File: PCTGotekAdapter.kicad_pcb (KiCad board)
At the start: 2 copper layers, 114.3 x 55.9 mm, 21 parts, among them J1 Conn_02x17_Odd_Even, J2 Conn_2Rows-19Pins, J3 Conn_2Rows-19Pins, J4 Conn_02x17_Odd_Even, J5 Conn_01x04_Pin, J6 Conn_01x04_Pin, U1 SN74LS138N, U2 SN7407N

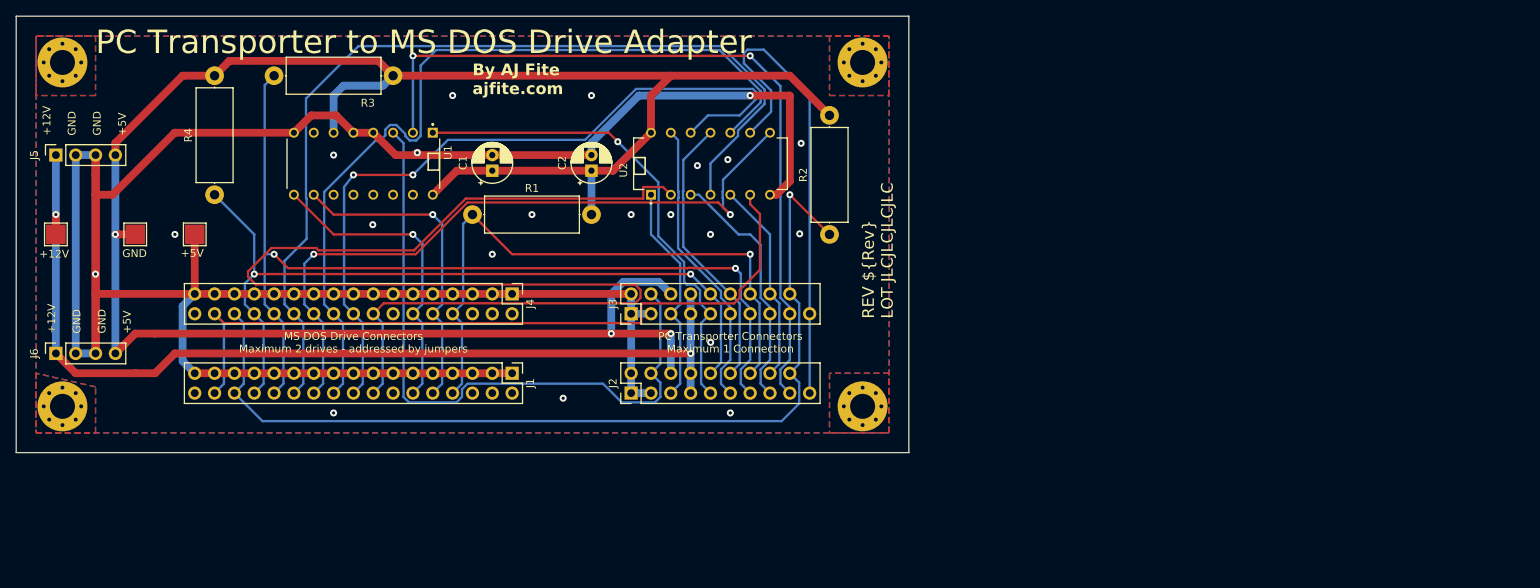
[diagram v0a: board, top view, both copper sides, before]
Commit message: First pass at REV B
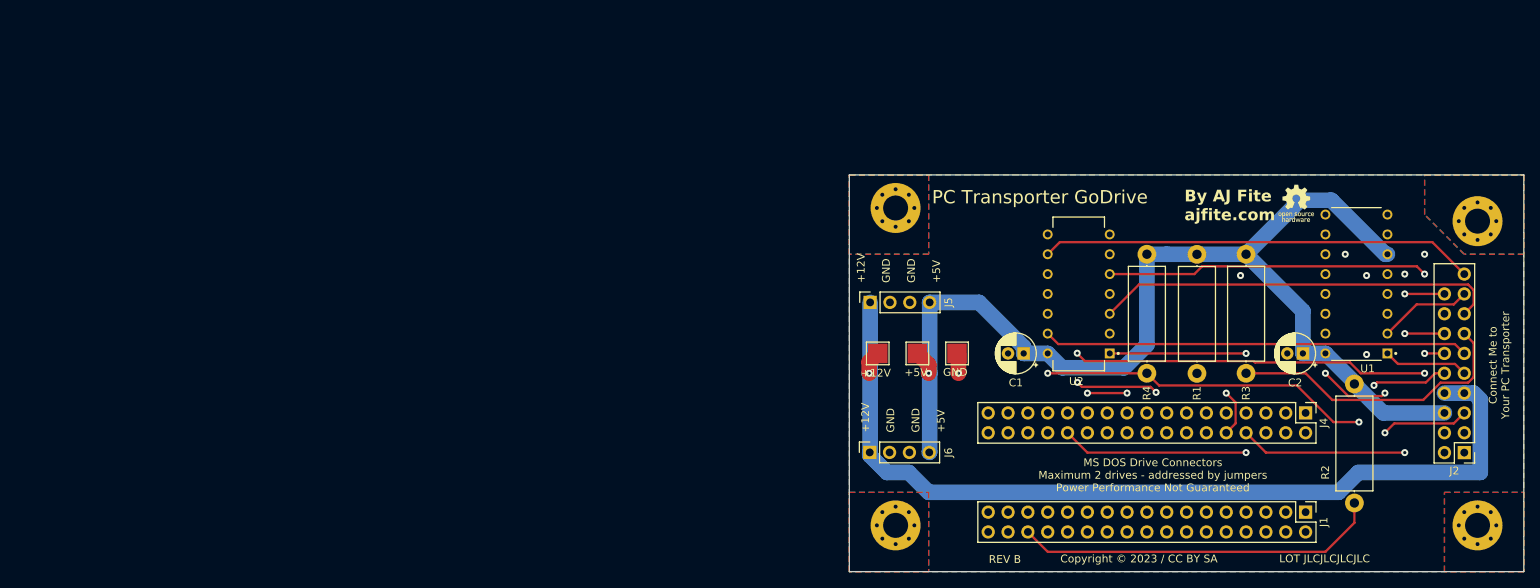
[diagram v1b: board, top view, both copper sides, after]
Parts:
- removed J3: Conn_2Rows-19Pins, Connector_PinHeader_2.54mm:PinHeader_2x10_P2.54mm_Vertical
- moved R3 130.2 mm to (175.3, 99.1), turned to 90 degrees
- moved U1 128.1 mm to (189.4, 87.6), turned to 180 degrees
- moved R4 121.5 mm to (162.6, 99.1)
- moved H1 108.3 mm to (130.4, 77.9)
- moved H2 107.8 mm to (130.4, 118.5)
- moved J2 107.0 mm to (203.2, 109.2), turned to 180 degrees
- moved TP1 106.3 mm to (128.1, 96.5)
- moved J5 106.0 mm to (127.1, 90.0)
- moved J6 105.0 mm to (127.1, 109.2)
- moved J1 103.1 mm to (182.9, 116.8)
- moved J4 102.7 mm to (182.9, 104.1)
- moved TP2 101.3 mm to (133.2, 96.5)
- moved TP3 98.8 mm to (138.2, 96.5)
- moved R1 95.0 mm to (169.0, 99.1), turned to 90 degrees
- moved C2 94.1 mm to (182.5, 96.5), turned to 180 degrees
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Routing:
- net +5V: track 278.0 -> 140.7 mm, vias 3 -> 1
- net Net-(J1-Pin_16): track 159.0 -> 31.6 mm
- net Net-(J1-Pin_24): track 120.5 -> 32.7 mm
- net Net-(J2-Pin_17): track 99.3 -> 11.9 mm, vias 2 -> 0
- net Net-(J1-Pin_20): track 107.3 -> 42.2 mm, vias 0 -> 2
- net Net-(J2-Pin_4): track 85.1 -> 21.1 mm
- net Net-(J1-Pin_18): track 97.3 -> 40.3 mm
- net Net-(J2-Pin_9): track 62.9 -> 10.9 mm, vias 1 -> 0
- net Net-(J1-Pin_32): track 96.4 -> 45.9 mm
- net Net-(J1-Pin_26): track 121.4 -> 86.7 mm, vias 2 -> 1
- net Net-(J1-Pin_22): track 89.9 -> 55.9 mm, vias 2 -> 0
- net Net-(J2-Pin_5): track 28.4 -> 54.0 mm, vias 0 -> 4
- net Net-(J1-Pin_30): track 121.3 -> 97.1 mm
- net Net-(J2-Pin_12): track 35.8 -> 59.9 mm, vias 0 -> 3
- net Net-(J2-Pin_16): track 26.0 -> 47.3 mm, vias 0 -> 1
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- added copper zone on In1.Cu, net GND
- added copper zone on In2.Cu, net GND
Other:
- board size 114.3 x 55.9 mm -> 86.4 x 50.8 mm
- copper layers 2 -> 4
- board text added: "Connect Me to Your PC Transporter"
- board text added: "Copyright ©️ 2023 / CC BY SA"
- board text added: "LOT JLCJLCJLCJLC"
- board text added: "MS DOS Drive Connectors Maximum 2 drives - addressed by jumpers Power Performance Not Guaranteed"
- board text added: "PC Transporter GoDrive"
- board text added: "REV B"
- board text removed: "MS DOS Drive Connectors Maximum 2 drives - addressed by jumpers"
- board text removed: "PC Transporter Connectors Maximum 1 Connection"
- board text removed: "PC Transporter to MS DOS Drive Adapter"
- board text removed: "REV ${Rev} LOT JLCJLCJLCJLC"
